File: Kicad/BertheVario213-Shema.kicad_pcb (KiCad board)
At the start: 2 copper layers, 42.5 x 109 mm, 15 parts, among them Q1 S8050, SW1 Gauche, SW2 Centre, SW3 Droit

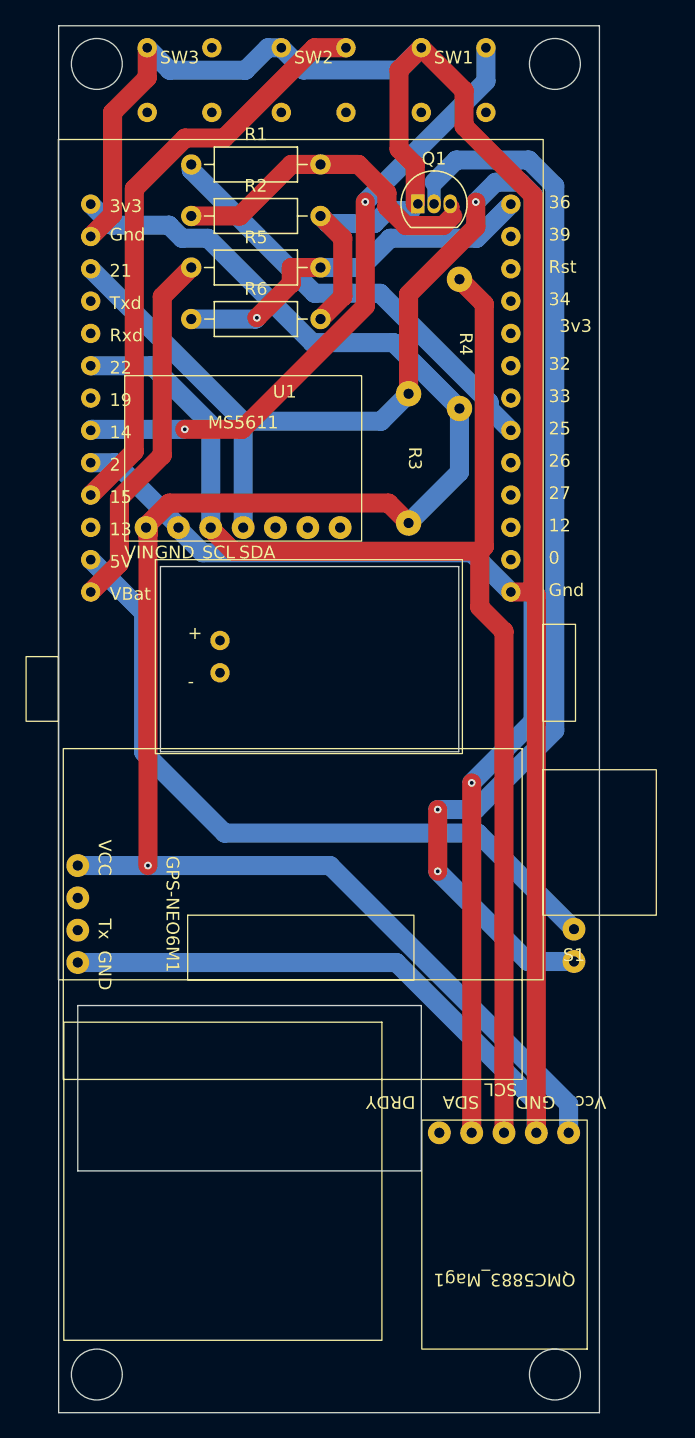
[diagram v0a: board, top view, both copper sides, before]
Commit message: modif pcb
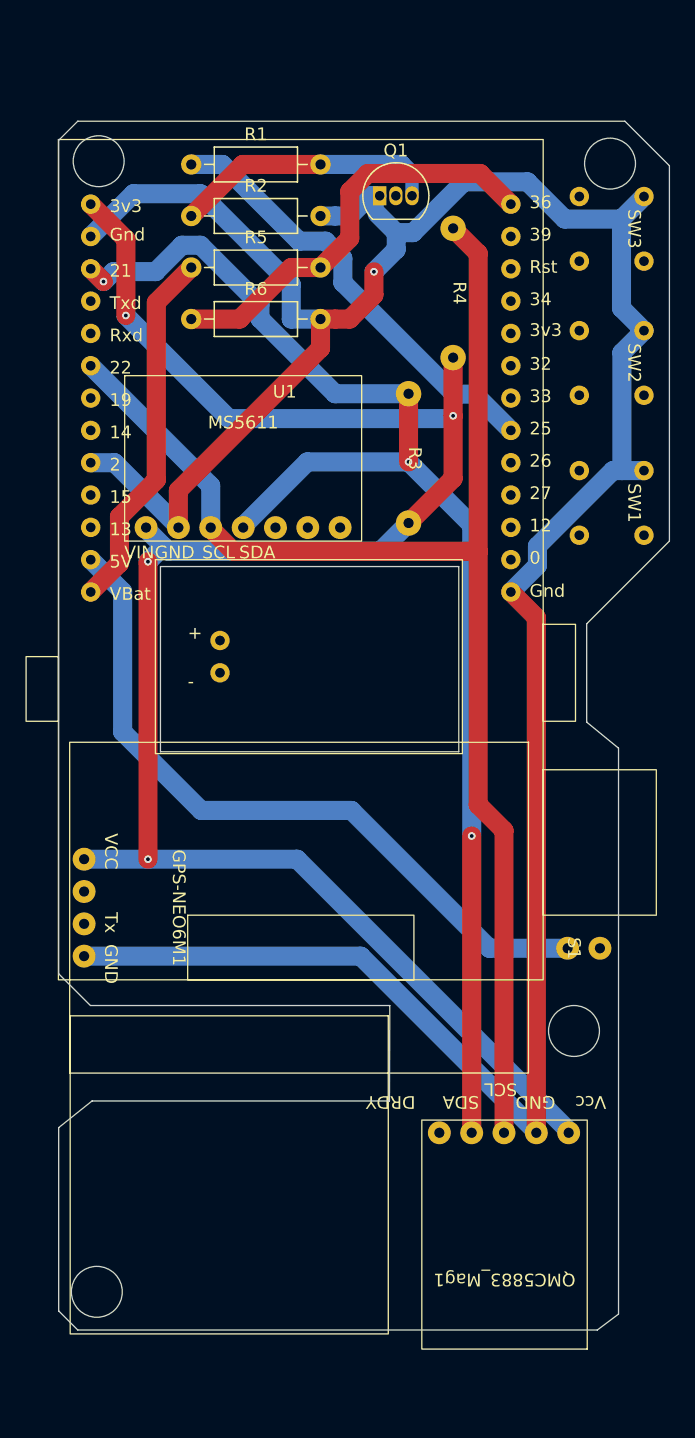
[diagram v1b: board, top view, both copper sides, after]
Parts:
- moved SW3 37.5 mm to (167.2, 76.0), turned to -90 degrees
- moved SW1 37.1 mm to (167.2, 97.5), turned to -90 degrees
- moved SW2 34.1 mm to (167.2, 86.5), turned to -90 degrees
- moved R4 4.03 mm to (153.5, 81.0)
- moved Q1 3.07 mm to (147.7, 73.4)
- moved S1 1.15 mm to (162.5, 132.5), turned to -90 degrees
- moved GPS-NEO6M1 0.71 mm to (126.4, 129.3)
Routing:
- net Net-(Q1-C): track 85.8 -> 0.00 mm, vias 2 -> 0
- net Net-(U1-Bouton_Gauche): track 49.9 -> 0.00 mm, vias 2 -> 0
- net Net-(U1-Bouton_Centre): track 46.7 -> 0.00 mm
- net Net-(MS5611-SDA): track 137.7 -> 107.4 mm, vias 2 -> 3
- net GNDREF: track 244.0 -> 219.0 mm, vias 0 -> 1
- net Net-(Q1-B): track 26.2 -> 21.0 mm
- net Net-(GPS-NEO6M1-VCC): track 144.1 -> 148.1 mm, vias 1 -> 4
- net Net-(U1-In_Vbat): track 29.6 -> 33.0 mm, vias 1 -> 0
- net Net-(MS5611-SCL): track 110.2 -> 111.2 mm
- net Net-(U1-Speaker): track 34.3 -> 34.9 mm
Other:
- board size 42.5 x 109 mm -> 48 x 95 mm
